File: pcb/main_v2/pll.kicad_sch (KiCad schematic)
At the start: 52 parts, among them U601 ADF4351, U602 XMB0220K1-50100G, U603 PD0922J5050D2HF, Y601 ATX-11-F-26.000MHZ-F05-T

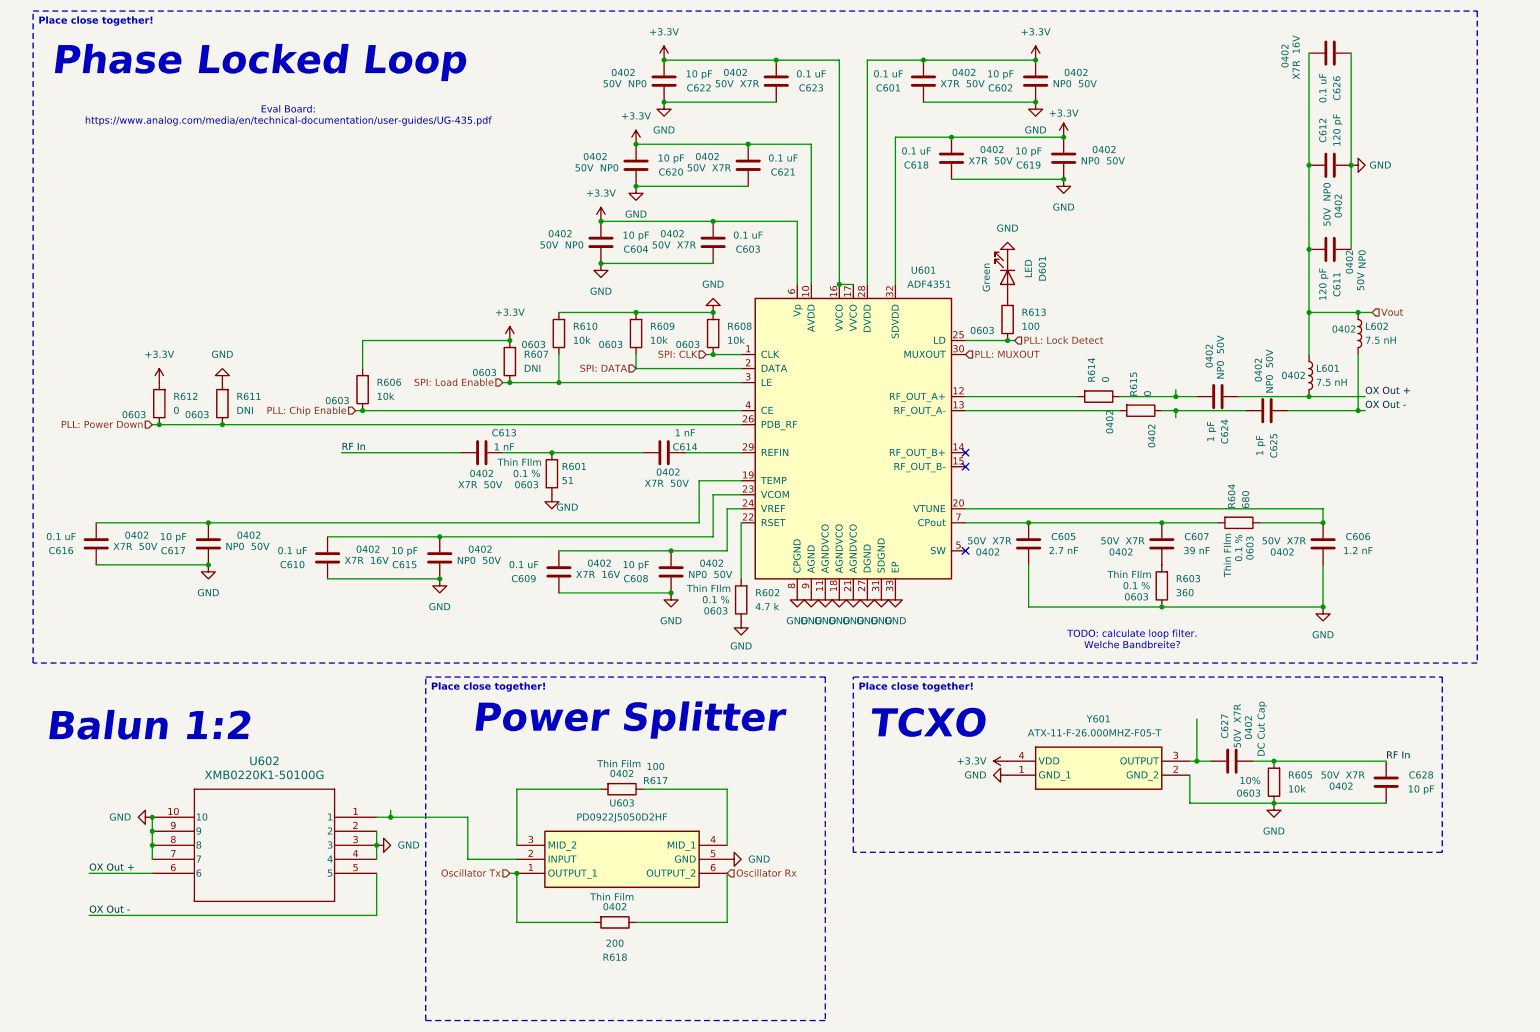
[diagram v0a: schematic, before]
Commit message: updarted schematic and simulation
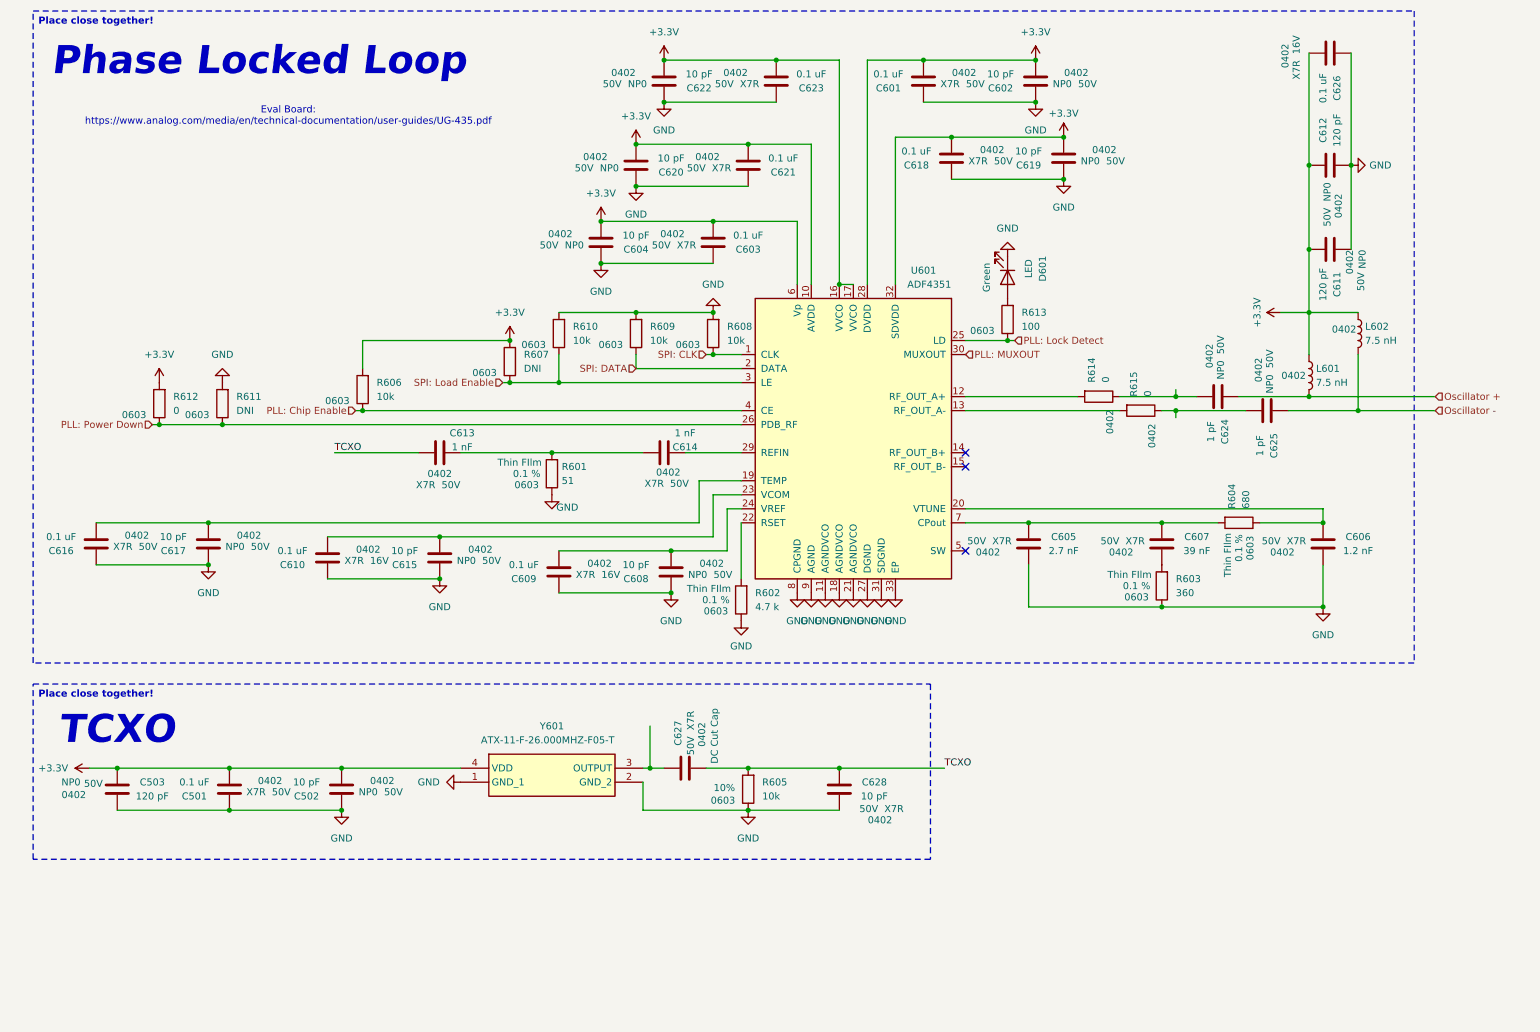
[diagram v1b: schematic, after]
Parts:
- removed R617: 100, Resistor_SMD:R_0402_1005Metric, symbol Device:R
- removed R618: 200, Resistor_SMD:R_0402_1005Metric, symbol Device:R
- removed U602: XMB0220K1-50100G, My Footprints:XMB0220K1-50100G_TTT, symbol My Symbols:XMB0220K1-50100G
- removed U603: PD0922J5050D2HF, PD0922J5050D2HF, symbol My Symbols:PD0922J5050D2HF
- added C501: 0.1 uF, Capacitor_SMD:C_0402_1005Metric, symbol Device:C
- added C502: 10 pF, Capacitor_SMD:C_0402_1005Metric, symbol Device:C
- added C503: 120 pF, Capacitor_SMD:C_0402_1005Metric, symbol Device:C
- Y601: footprint ATX11F26000MHZF05T -> My Footprints:ATX11F26000MHZF05T
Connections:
- net Vout is gone; now on net +3.3V: C611.1, C612.2, C626.1, L601.1, L602.1
- net +3.3V: now also C501.1, C502.1, C503.2
- net GND: now also C501.2, C502.2, C503.1
- net OX Out + renamed Oscillator +
- net OX Out - renamed Oscillator -
- net RF In renamed TCXO
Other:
- note removed: "Balun 1:2"
- note removed: "Power Splitter"
- note removed: "TODO: calculate loop filter. Welche Bandbreite?"
- moved on the sheet: C613, C627, C628, R605, Y601
